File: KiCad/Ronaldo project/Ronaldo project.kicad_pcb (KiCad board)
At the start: 2 copper layers, 45.7 x 69.2 mm, 24 parts, among them J1 Power, J2 Program, J3 RFID Module, J4 Coin Acceptor, M1 Motor_DC, M2 Motor_DC, SW1 Switch, SW2 Reset, SW3 SW_Push, SW4 SW_Push, U1 L293D, U3 ESP-12E, U4 AMS1117-3.3, U5 TSOP41xx

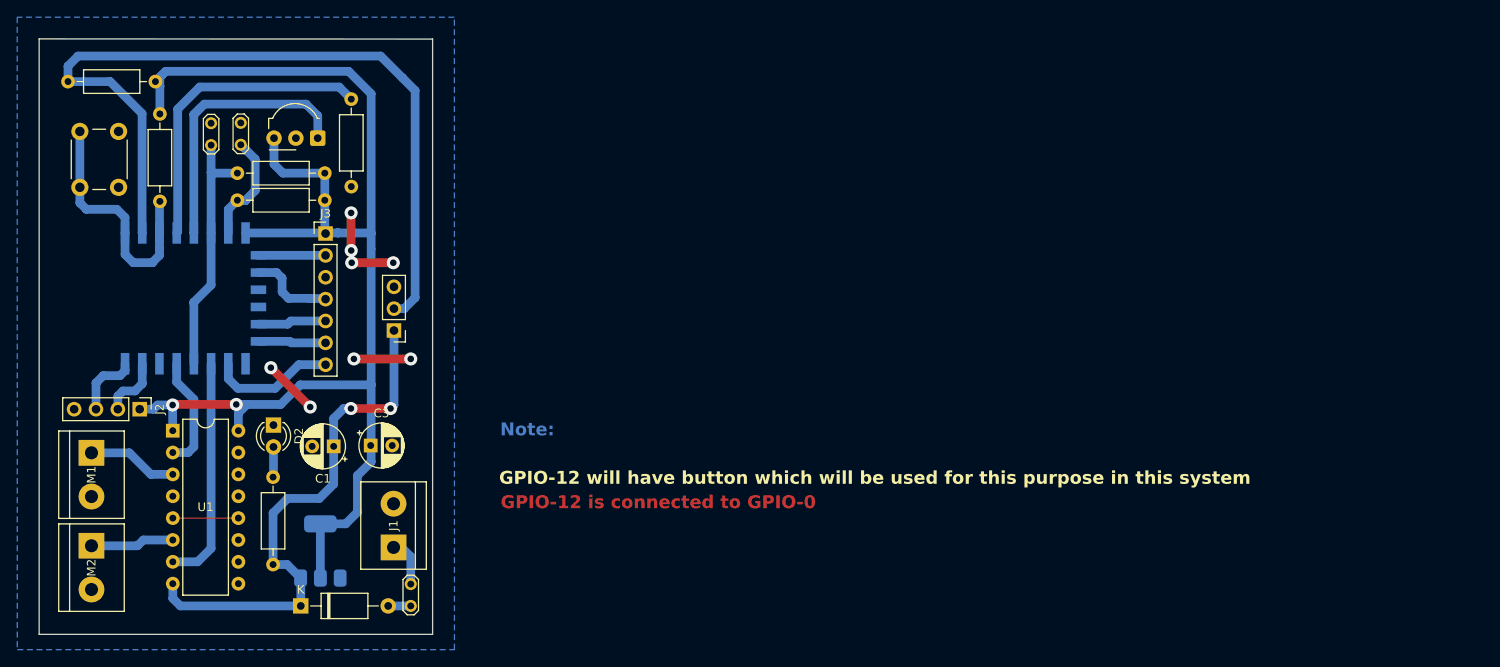
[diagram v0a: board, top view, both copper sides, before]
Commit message: Updates
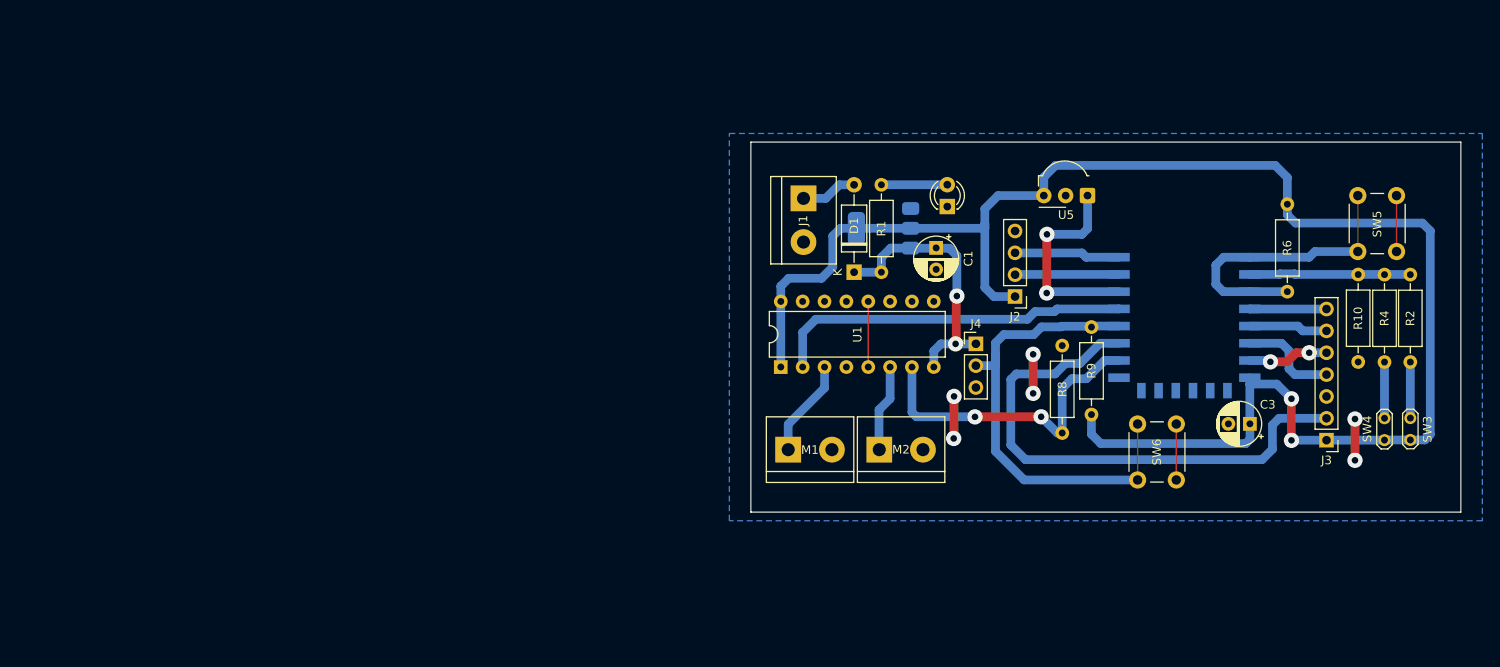
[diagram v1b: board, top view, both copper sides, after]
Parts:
- removed R3, R5, R7: 10k, Resistor_THT:R_Axial_DIN0207_L6.3mm_D2.5mm_P10.16mm_Horizontal
- removed SW1: Switch, TestPoint:TestPoint_2Pads_Pitch2.54mm_Drill0.8mm
- removed SW2: Reset, Button_Switch_THT:SW_PUSH_6mm
- removed U3: ESP-12E, RF_Module:ESP-12E
- added R10: 10k, Resistor_THT:R_Axial_DIN0207_L6.3mm_D2.5mm_P10.16mm_Horizontal, F.Cu at (205.6, 96.5)
- added R6: 10k, Resistor_THT:R_Axial_DIN0207_L6.3mm_D2.5mm_P10.16mm_Horizontal, F.Cu at (197.3, 88.4)
- added R8: 10k, Resistor_THT:R_Axial_DIN0207_L6.3mm_D2.5mm_P10.16mm_Horizontal, F.Cu at (171.2, 104.8)
- added R9: 10k, Resistor_THT:R_Axial_DIN0207_L6.3mm_D2.5mm_P10.16mm_Horizontal, F.Cu at (174.6, 102.7)
- added SW5: Reset, Button_Switch_THT:SW_PUSH_6mm, F.Cu at (210.0, 77.2)
- added SW6: Mode, Button_Switch_THT:SW_PUSH_6mm, F.Cu at (179.9, 110.3)
- added U2: ESP-12F, RF_Module:ESP-12E, B.Cu at (185.4, 87.9)
- D1: value D_Small -> 1N4001
- J4: value Coin Acceptor -> Coin
- R2: value 10k -> 22k
- R4: value 10k -> 47k
- SW3: value SW_Push -> BTN1
- SW4: value SW_Push -> BTN2
- moved SW3 143.5 mm to (211.6, 103.1)
- moved SW4 137.9 mm to (208.6, 105.6), turned to 90 degrees
- moved R2 126.4 mm to (211.6, 86.4), turned to -90 degrees
- moved R4 123.7 mm to (208.6, 86.4), turned to -90 degrees
- moved J3 118.8 mm to (201.9, 105.6), turned to 180 degrees
- moved J2 102.6 mm to (165.7, 89.0), turned to 180 degrees
- moved C3 102.2 mm to (193.0, 103.7), turned to 180 degrees
- moved M2 92.2 mm to (149.9, 106.7), turned to 0 degrees
- moved U5 89.7 mm to (174.1, 77.2)
- moved D2 82.3 mm to (157.8, 78.5), turned to 90 degrees
- moved M1 81.0 mm to (139.3, 106.7), turned to 0 degrees
- moved R1 78.4 mm to (150.2, 86.1)
- moved U4 75.4 mm to (150.4, 81.0), turned to 180 degrees
- moved D1 75.1 mm to (147.0, 86.1), turned to 90 degrees
- moved C1 73.7 mm to (156.5, 83.3), turned to -90 degrees
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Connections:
- J1 pad 1: Net-(J1-Pin_1) -> Net-(D1-A)
- J2 pad 2: /Rx -> /RXD
- J2 pad 3: /Tx -> /TXD
- R2 pad 1: +3V3 -> Net-(U2-ADC)
- R2 pad 2: /button2 -> Net-(R2-Pad2)
- R4 pad 1: +3V3 -> Net-(U2-ADC)
- R4 pad 2: /button1 -> Net-(R4-Pad2)
- SW3 pad 1: GND -> Net-(R2-Pad2)
- SW3 pad 2: /button1 -> +3V3
- SW4 pad 1: GND -> +3V3
- SW4 pad 2: /button2 -> Net-(R4-Pad2)
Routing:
- net /RST: track 7.80 -> 63.0 mm
- net /coin: track 95.4 -> 55.8 mm
- net Net-(U3-GPIO16): track 36.3 -> 0.00 mm
- net Net-(SW5A-D): track 0.00 -> 34.5 mm
- net +3V3: track 158.0 -> 191.4 mm
- net +12V: track 62.4 -> 31.9 mm
- net Net-(SW2A-C): track 29.7 -> 0.00 mm
- net /button1: track 29.3 -> 0.00 mm
- net /motor1: track 13.2 -> 41.9 mm
- net Net-(U2-ADC): track 0.00 -> 18.7 mm
- net /button2: track 12.9 -> 0.00 mm
- net /TXD: track 0.00 -> 12.3 mm
- net /RXD: track 0.00 -> 12.1 mm
- net /motor2: track 26.5 -> 36.9 mm, vias 0 -> 2
- net Net-(U2-GPIO5): track 33.1 -> 24.1 mm, vias 0 -> 2
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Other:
- board size 45.7 x 69.2 mm -> 82.5 x 43 mm
- board text removed: "GPIO-12 is connected to GPIO-0"
- board text removed: "GPIO-12 will have button which will be used for this purpose in this system"
- board text removed: "In this body mode is seted using GPIO-12"
- board text removed: "Note:"
